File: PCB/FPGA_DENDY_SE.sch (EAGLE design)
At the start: 140 parts, among them CN1 DENDY60PINSLOT, J1 NTSC/PAL, J2 DENDY, Q1 14.318 MHz, Q2 17.734 MHz, U1 EP1C3T100C8N, U10 OPA2134U, U11 SN74LVC2G34DBVR, U12 THS7314DR, U13 74LS373WMSO20, U14 SN74LVC1G125DBVR, U15 74LVC1G04GV, U16 SN74LVC1G3157, U2 EPCS4, U3 SN74LVC8T245, U4 SN74LVC8T245, U5 SN74LVC1G240DBVR, U6 SN74LVC1G240DBVR, U7 SN74LVC1G240DBVR, U8 SN74LVC1G240DBVR, X1 057-010-1

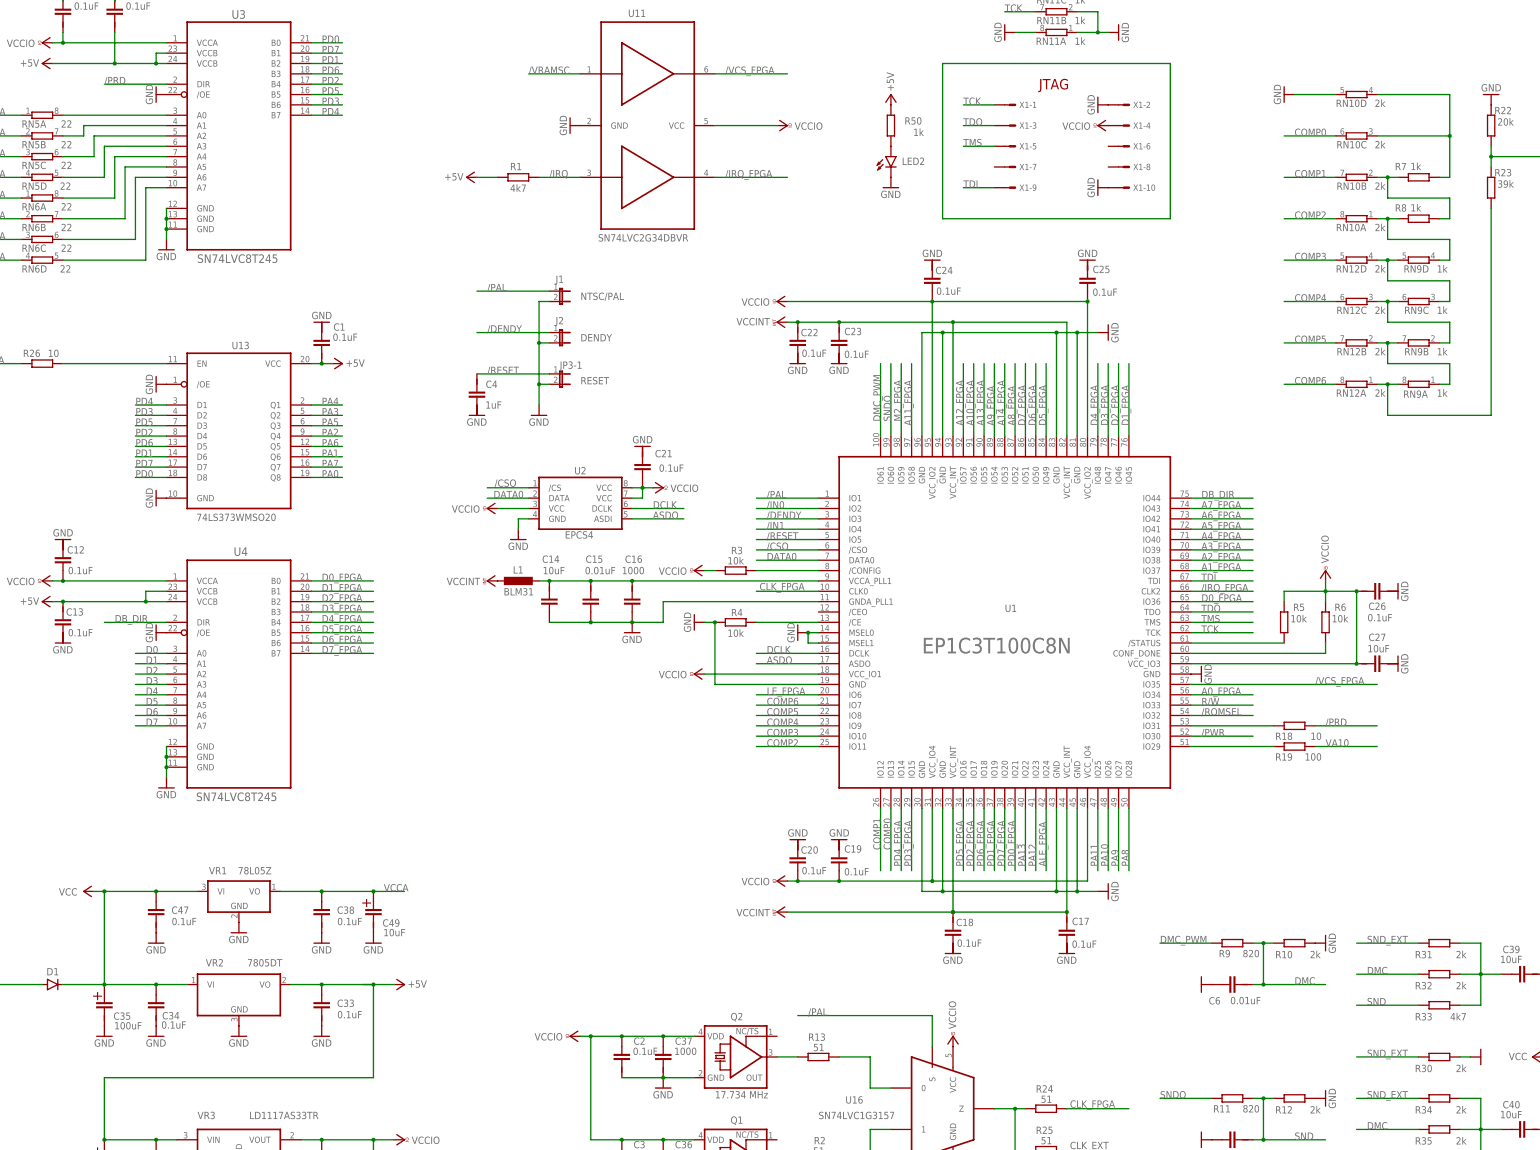
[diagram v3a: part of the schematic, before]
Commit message: Add files via upload
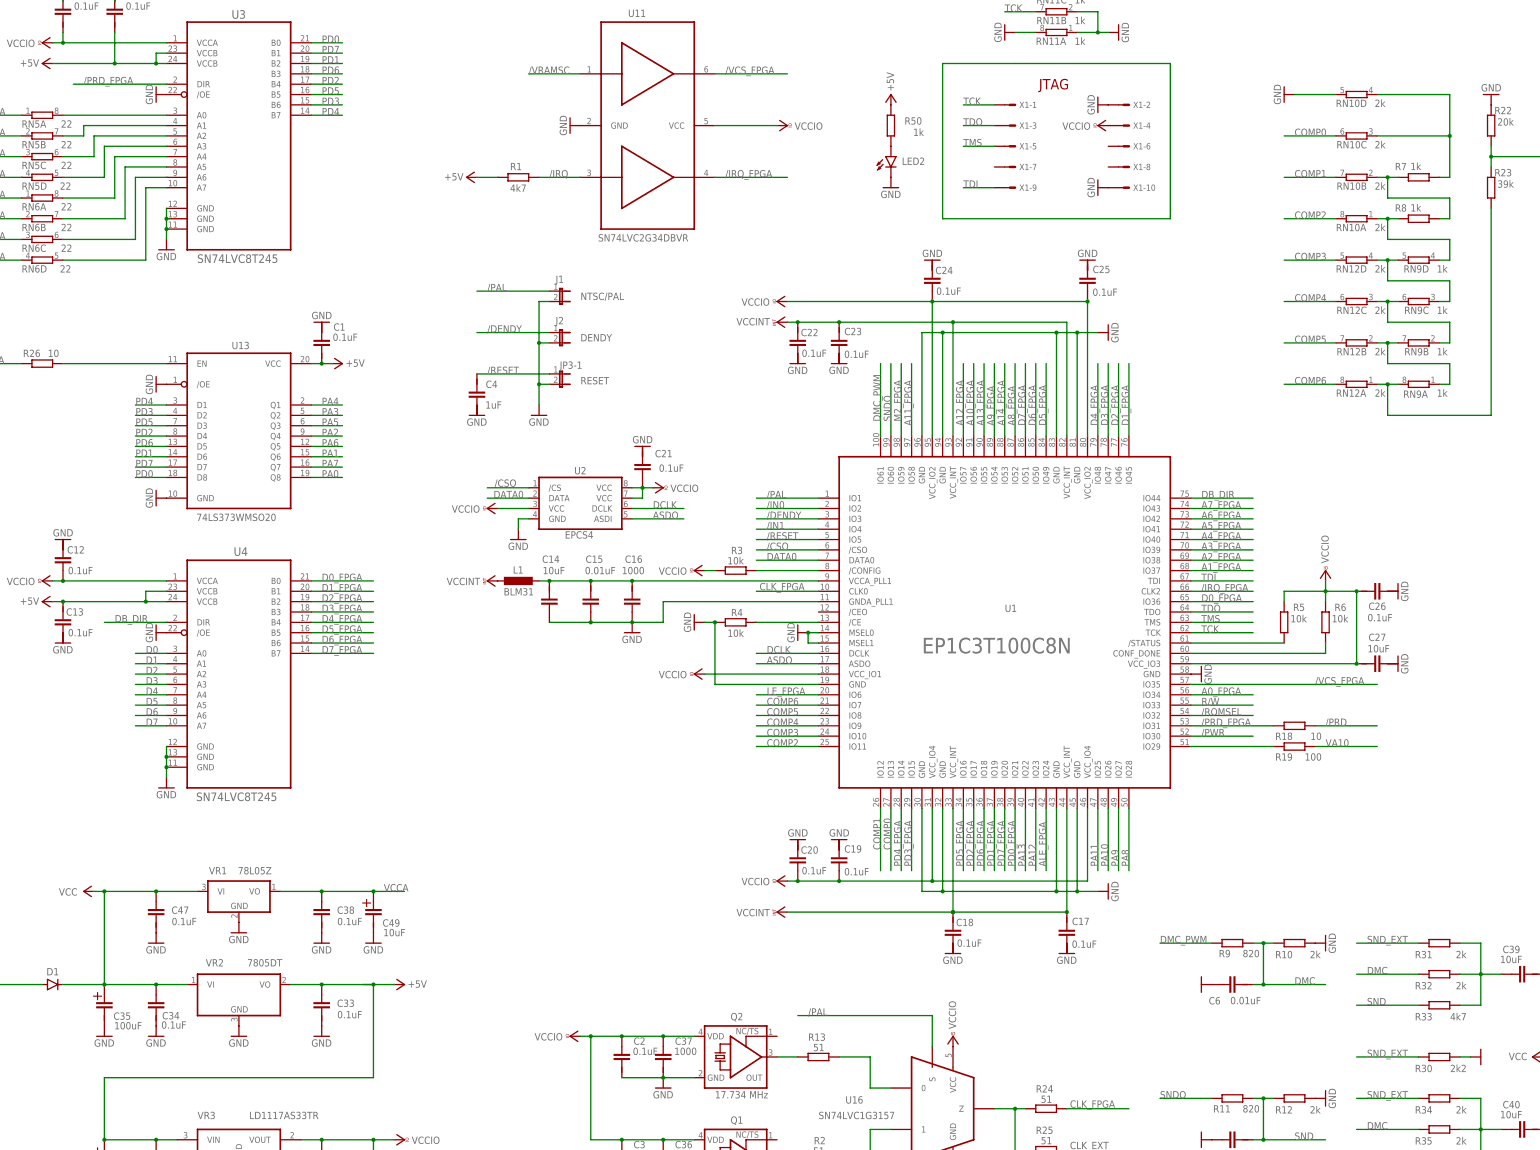
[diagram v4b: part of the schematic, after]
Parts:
- R30: value 2k -> 2k2
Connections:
- net N$14 renamed /PWR_FPGA
- removed net N$13: R18.1, U1.IO31
- new net /PRD_FPGA: R18.1, U1.IO31, U3.DIR
- net /PRD: no longer U3.DIR
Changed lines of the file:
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@@
 <part name="C5" library="rcl_my" deviceset="C-EU" device="C0805" package3d_urn="urn:adsk.eagle:package:23617/2" value="0.01uF"/>
 <part name="GND48" library="supply1" library_urn="urn:adsk.eagle:library:371" deviceset="GND" device=""/>
-<part name="R30" library="rcl" library_urn="urn:adsk.eagle:library:334" deviceset="R-EU_" device="R0805" package3d_urn="urn:adsk.eagle:package:23553/2" value="2k"/>
+<part name="R30" library="rcl" library_urn="urn:adsk.eagle:library:334" deviceset="R-EU_" device="R0805" package3d_urn="urn:adsk.eagle:package:23553/2" value="2k2"/>
 <part name="GND76" library="supply1" library_urn="urn:adsk.eagle:library:371" deviceset="GND" device=""/>
 <part name="GND49" library="supply1" library_urn="urn:adsk.eagle:library:371" deviceset="GND" device=""/>
@@
 <net name="/PRD" class="0">
 <segment>
-<pinref part="U3" gate="G$1" pin="DIR"/>
-<wire x1="-205.74" y1="129.54" x2="-220.98" y2="129.54" width="0.1524" layer="91"/>
-<label x="-220.98" y="129.54" size="1.778" layer="95"/>
-</segment>
-<segment>
 <wire x1="-350.52" y1="0" x2="-342.9" y2="0" width="0.1524" layer="91"/>
 <pinref part="CN1" gate="G$1" pin="/PRD"/>
@@
 </segment>
 </net>
-<net name="N$13" class="0">
+<net name="/PRD_FPGA" class="0">
 <segment>
 <pinref part="R18" gate="G$1" pin="1"/>
 <pinref part="U1" gate="G$1" pin="IO31"/>
 <wire x1="66.04" y1="-27.94" x2="45.72" y2="-27.94" width="0.1524" layer="91"/>
+<label x="48.26" y="-27.94" size="1.778" layer="95"/>
+</segment>
+<segment>
+<pinref part="U3" gate="G$1" pin="DIR"/>
+<wire x1="-205.74" y1="129.54" x2="-228.6" y2="129.54" width="0.1524" layer="91"/>
+<label x="-226.06" y="129.54" size="1.778" layer="95"/>
 </segment>
 </net>
-<net name="N$14" class="0">
+<net name="/PWR_FPGA" class="0">
 <segment>
 <pinref part="R19" gate="G$1" pin="1"/>

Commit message: Add files via upload
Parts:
- removed C59, C60, C61, C62: 0.1uF, rcl_my:C-EUC0805
- removed R50, R63: 1k, rcl:R-EU_R0805
- removed R67: 10, rcl:R-EU_R0805
- removed U16: SN74LVC1G3157, SN74LVC1G3157:SN74LVC1G3157
- added C51, C52, C54: 10uF, rcl_my:CPOL-EU153CLV-0505
- added C53: 0.1uF, rcl_my:C-EUC0805
- added C7: 0.1uF, rcl_my:C-EUC0603
- added R27, R28: 2k, rcl:R-EU_R0805
- added R29: 4k7, rcl:R-EU_R0805
- added U9: THS7314DR, THS7314DR:THS7314
- C10: value 0.1uF -> 10uF; device rcl_my:C-EUC0805 -> rcl_my:CPOL-EU153CLV-0505
- C11: value 220uF -> 100uF
- C12, C13, C17, C18, C50, C8: device rcl_my:C-EUC0603 -> rcl_my:C-EUC0805
- C14: value 10uF -> 100uF; device rcl_my:C-EUC0603 -> rcl_my:CPOL-EU153CLV-0505
- C15: value 0.01uF -> 0.1uF; device rcl_my:C-EUC0603 -> rcl_my:C-EUC0805
- C16: value 1000 -> 0.1uF; device rcl_my:C-EUC0603 -> rcl_my:C-EUC0805
- C19: value 0.1uF -> 22uF; device rcl_my:C-EUC0603 -> rcl_my:CPOL-EU153CLV-0505
- C26: value 0.1uF -> 10uF
- C27: value 10uF -> 0.01uF
- C28: value 0.1uF -> 1000; device rcl_my:C-EUC0805 -> rcl_my:C-EUC0603
- C29: value 0.1uF -> 1uF; device rcl_my:C-EUC0805 -> rcl_my:C-EUC0603
- C30, C31, C33, C38, C40, C45: device rcl_my:C-EUC0805 -> rcl_my:C-EUC0603
- C32: value 22uF -> 0.1uF; device rcl_my:CPOL-EU153CLV-0505 -> rcl_my:C-EUC0603
- C35: value 100uF -> 1000; device rcl_my:CPOL-EU153CLV-0505 -> rcl_my:C-EUC0805
- C36: value 1000 -> 0.1uF
- C39: value 10uF -> 0.1uF; device rcl_my:C-EUC0805 -> rcl_my:C-EUC0603
- C4: value 1uF -> 0.1uF; device rcl_my:C-EUC0603 -> rcl_my:C-EUC0805
- C41, C42: value 0.1uF -> 0.01uF
- C43: value 10uF -> 0.1uF; device rcl_my:CPOL-EU153CLV-0505 -> rcl_my:C-EUC0603
- C44: value 10uF -> 220uF
- C46: value 10uF -> 0.1uF
- C48: value 0.1uF -> 10uF; device rcl_my:C-EUC0603 -> rcl_my:C-EUC0805
- C49: device rcl_my:CPOL-EU153CLV-0505 -> rcl_my:C-EUC0805
- C5: value 0.01uF -> 0.1uF
- C6: value 0.01uF -> 0.1uF; device rcl_my:C-EUC0805 -> rcl_my:C-EUC0603
- C9: value 100uF -> 0.1uF; device rcl_my:CPOL-EU153CLV-0505 -> rcl_my:C-EUC0805
- R1: value 4k7 -> 10
- R10: value 2k -> 51
- R11: value 820 -> 1k
- R12: value 2k -> 1k
- R13: value 51 -> 20k
- R14: value 10k -> 39k
- R17: value 10k -> 10
- R18: value 10 -> 100
- R19: value 100 -> 820
- R2: value 51 -> 10
- R20: value 10 -> 2k
- R21: value 75 -> 820
- R22: value 20k -> 2k
- R23: value 39k -> 2k
- R24: value 51 -> 2k
- R25: value 51 -> 4k7
- R26: value 10 -> 2k2
- R3: value 10k -> 4k7
- R30: value 2k2 -> 75
- R31, R32, R34: value 2k -> 10k
- R33: value 4k7 -> 10k
- R35: value 2k -> 10
- R36, RN8: value 4k7 -> 1k
- R4: value 10k -> 1k
- R7, R8: value 1k -> 51
- R9: value 820 -> 51
- RN12: value 2k -> 4k7
- RN9: value 1k -> 2k
- U10: value OPA2134U -> SN74LVC1G125DBVR; device burr-brown:OPA2134U -> SN74LVC1G125DBVR:SN74LVC1G125DBVR
- U11: value SN74LVC2G34DBVR -> SN74LVC1G240DBVR; device SN74LVC2G34DBVR:SN74LVC2G34DBVR -> SN74LVC1G240DBVR:SN74LVC1G240DBVR
- U12: value THS7314DR -> SN74LVC1G240DBVR; device THS7314DR:THS7314 -> SN74LVC1G240DBVR:SN74LVC1G240DBVR
- U13: value 74LS373WMSO20 -> SN74LVC1G240DBVR; device 74LS373WM:74LS373WMSO20 -> SN74LVC1G240DBVR:SN74LVC1G240DBVR
- U14: value SN74LVC1G125DBVR -> SN74LVC1G240DBVR; device SN74LVC1G125DBVR:SN74LVC1G125DBVR -> SN74LVC1G240DBVR:SN74LVC1G240DBVR
- U15: value 74LVC1G04GV -> OPA2134U; device 74LVC1G04GV:74LVC1G04GV -> burr-brown:OPA2134U
- U2: value EPCS4 -> SN74LVC8T245; device EPCS4:EPCS4 -> SnapEDA-Library:SN74LVC8T245
- U3: value SN74LVC8T245 -> 74LS373WMSO20; device SnapEDA-Library:SN74LVC8T245 -> 74LS373WM:74LS373WMSO20
- U5: value SN74LVC1G240DBVR -> SN74LVC2G34DBVR; device SN74LVC1G240DBVR:SN74LVC1G240DBVR -> SN74LVC2G34DBVR:SN74LVC2G34DBVR
- U6: value SN74LVC1G240DBVR -> 74LVC1G04GV; device SN74LVC1G240DBVR:SN74LVC1G240DBVR -> 74LVC1G04GV:74LVC1G04GV
- U7: value SN74LVC1G240DBVR -> EPCS4; device SN74LVC1G240DBVR:SN74LVC1G240DBVR -> EPCS4:EPCS4
- U8: value SN74LVC1G240DBVR -> SN74LVC1G3157; device SN74LVC1G240DBVR:SN74LVC1G240DBVR -> SN74LVC1G3157:SN74LVC1G3157
- renumbered R61 to R39, R62 to R40, R64 to R41, R65 to R37, R66 to R42, R68 to R38
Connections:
- net +5V: now also C13.1, C14.+, C15.1, C2.1, C20.2, C4.2, C45.2, C46.1, C47.1, C5.2, C7.2, R3.1, R31.1, R32.1, R33.1, R34.1, R4.2, U10.VCC, U11.VCC, U12.VCC, U2.VCCB@1, U2.VCCB@2, U3.VCC; no longer C10.2, C13.2, C28.1, C33.1, C50.2, C59.2, C60.1, C61.1, C62.1, C8.2, C9.+, R1.1, R14.1, R15.1, R16.1, R17.1, R50.2, U15.VCC, U3.VCCB@1, U3.VCCB@2, U5.VCC, U7.VCC, U8.VCC
- net /CSO: now also U7./CS; no longer U2./CS
- net /IN0: now also U11./OE, U13./OE; no longer U6./OE, U8./OE
- net /IN1: now also U12./OE, U14./OE; no longer U5./OE, U7./OE
- net /IRQ: now also R3.2, U5.IN2; no longer R1.2, U11.IN2
- net /IRQ_FPGA: now also U5.OUT2; no longer U11.OUT2
- net /PA13: now also U6.OUT; no longer U15.OUT
- net /PAL: now also U8.S; no longer U16.S
- net /PRD: now also R17.2; no longer R18.2
- net /PRD_FPGA: now also R17.1, U2.DIR; no longer R18.1, U3.DIR
- net /PWR_FPGA: now also R18.1; no longer R19.1
- net /RESET: now also C29.2; no longer C4.2
- net /VCS_FPGA: now also U5.OUT1; no longer U11.OUT1
- net /VRAMSC: now also U5.IN1; no longer U11.IN1
- net ALE_FPGA: now also R2.1; no longer R26.1
- net ASDO: now also U7.ASDI; no longer U2.ASDI
- net CLK_EXT: now also R10.2; no longer R25.2
- net CLK_FPGA: now also R9.2; no longer R24.2
- net COMP0: now also RN9C.2; no longer RN10C.2
- net COMP1: now also RN9B.2; no longer RN10B.2
- net COMP2: now also RN9A.2; no longer RN10A.2
- net COMP3: now also RN10D.2; no longer RN12D.2
- net COMP4: now also RN10C.2; no longer RN12C.2
- net COMP5: now also RN10B.2; no longer RN12B.2
- net COMP6: now also RN10A.2; no longer RN12A.2
- net D0: now also U13.Y, U14.Y; no longer U5.Y, U6.Y
- net DATA0: now also U7.DATA; no longer U2.DATA
- net DCLK: now also U7.DCLK; no longer U2.DCLK
- net DMC: now also C41.2, R19.2, R20.1, R24.1, R28.1; no longer C6.2, R10.1, R32.1, R35.1, R9.2
- net DMC_PWM: now also R19.1; no longer R9.1
- net GND: now also C10.-, C11.-, C12.2, C13.2, C14.-, C15.2, C16.2, C17.2, C18.2, C26.1, C27.1, C28.1, C35.2, C42.1, C53.2, C54.-, C8.2, C9.2, R13.2, R20.2, R26.2, R6.1, RN12A.1, RN12D.1, RN8A.2, RN8B.1, RN9D.2, U10./OE, U15A.V-, U2./OE, U2.GND@1, U2.GND@2, U2.GND@3, U3.GND, U5.GND, U6.GND, U7.GND, U8.GND, U9.GND; no longer C10.1, C14.1, C15.1, C16.1, C2.2, C28.2, C29.2, C3.2, C30.2, C31.2, C33.2, C35.-, C38.2, C45.2, C49.-, C5.1, C6.1, C60.2, C61.2, C62.2, C9.-, R10.2, R12.2, R30.2, R4.1, RN10D.2, RN11A.1, RN11A.2, RN11B.1, RN8D.1, U10A.V-, U11.GND, U12.GND, U13./OE, U13.GND, U14./OE, U15.GND, U16.GND, U2.GND, U3.GND@1, U3.GND@2, U3.GND@3
- net JOYDATA1: now also R31.2, U13.A; no longer R14.2, U6.A
- net JOYDATA2: now also R33.2, U14.A; no longer R15.2, U5.A
- net LCH: now also C52.-; no longer C44.-
- net LE: now also U10.Y; no longer U14.Y
- net LE_FPGA: now also U10.A; no longer U14.A
- net M2_FPGA: now also U11.A, U12.A; no longer U7.A, U8.A
- net N$1: now also R15.1; no longer R5.1
- net N$10: now also R6.2; no longer R4.2
- net N$11: now also R5.2; no longer R3.2
- net N$12: now also C26.2, C27.2, C28.2; no longer C14.2, C15.2, C16.2
- net N$16: now also C48.1, R23.2, R24.2, R25.2; no longer C39.1, R31.2, R32.2, R33.2
- net N$17: now also R8.1; no longer R2.1
- net N$18: now also R7.1; no longer R13.1
- net N$19: now also U2.A1; no longer U3.A1
- net N$2: now also R16.1; no longer R6.1
- net N$20: now also U2.A2; no longer U3.A2
- net N$21: now also U2.A3; no longer U3.A3
- net N$22: now also U2.A4; no longer U3.A4
- net N$23: now also U2.A5; no longer U3.A5
- net N$24: now also U2.A6; no longer U3.A6
- net N$25: now also U2.A7; no longer U3.A7
- net N$26: now also R11.1, R12.2, RN9B.1; no longer R7.1, R8.2, RN10B.1
- net N$28: now also R14.1, RN10A.1, RN11A.2; no longer R23.1, RN12A.1, RN9A.2
- net N$30: now also C49.1, R27.2, R28.2, R29.2; no longer C40.1, R34.2, R35.2, R36.2
- net N$33: now also R1.1; no longer R20.1
- net N$34: now also R30.1, U9.CH3_OUT; no longer R21.1, U12.CH3_OUT
- net N$35: now also R7.2, U8.0; no longer R13.2, U16.0
- net N$36: now also C44.+, R30.2; no longer C11.+, R21.2
- net N$37: now also C51.+, R35.2; no longer C43.+, R67.2
- net N$38: now also C48.2, RN12C.1, RN12D.2, U15A.+IN; no longer C39.2, RN8C.1, RN8D.2, U10A.+IN
- net N$39: now also C49.2, RN12A.2, RN12B.1, U15B.+IN; no longer C40.2, RN8A.2, RN8B.1, U10B.+IN
- net N$4: now also RN10B.1, RN11A.1, RN11B.2; no longer RN12B.1, RN9A.1, RN9B.2
- net N$40: now also RN10D.1, RN11C.1, RN11D.2; no longer RN12D.1, RN9C.1, RN9D.2
- net N$41: now also R13.1, R14.2, U9.CH1_IN, U9.CH2_IN, U9.CH3_IN; no longer R22.1, R23.2, U12.CH1_IN, U12.CH2_IN, U12.CH3_IN
- net N$42: now also R36.2, U15A.-IN; no longer R63.2, U10A.-IN
- net N$43: now also R35.1, U15A.OUT; no longer R67.1, U10A.OUT
- net N$44: now also U15B.OUT; no longer U10B.OUT
- net N$45: now also U15B.-IN; no longer U10B.-IN
- net N$46: now also R8.2, U8.1; no longer R2.2, U16.1
- net N$47: now also R10.1, R9.1, U8.Z; no longer R24.1, R25.1, U16.Z
- net N$48: now also C52.+; no longer C44.+
- net N$5: now also R11.2, RN9C.1, RN9D.1; no longer R7.2, RN10C.1, RN10D.1
- net N$6: now also R2.2, U3.EN; no longer R26.2, U13.EN
- net N$63: now also R4.1; no longer R50.1
- net N$7: now also U2.A0; no longer U3.A0
- net N$8: now also R12.1, RN11D.1, RN9A.1; no longer R8.1, RN10A.1, RN9D.1
- net N$9: now also RN10C.1, RN11B.1, RN11C.2; no longer RN12C.1, RN9B.1, RN9C.2
- net PA0: now also U3.Q8; no longer U13.Q8
- net PA1: now also U3.Q6; no longer U13.Q6
- net PA12: now also R1.2; no longer R20.2
- net PA13: now also U6.IN; no longer U15.IN
- net PA2: now also U3.Q4; no longer U13.Q4
- net PA3: now also U3.Q2; no longer U13.Q2
- net PA4: now also U3.Q1; no longer U13.Q1
- net PA5: now also U3.Q3; no longer U13.Q3
- net PA6: now also U3.Q5; no longer U13.Q5
- net PA7: now also U3.Q7; no longer U13.Q7
- net PD0: now also U2.B0, U3.D8; no longer U13.D8, U3.B0
- net PD1: now also U2.B2, U3.D6; no longer U13.D6, U3.B2
- net PD2: now also U2.B4, U3.D4; no longer U13.D4, U3.B4
- net PD3: now also U2.B6, U3.D2; no longer U13.D2, U3.B6
- net PD4: now also U2.B7, U3.D1; no longer U13.D1, U3.B7
- net PD5: now also U2.B5, U3.D3; no longer U13.D3, U3.B5
- net PD6: now also U2.B3, U3.D5; no longer U13.D5, U3.B3
- net PD7: now also U2.B1, U3.D7; no longer U13.D7, U3.B1
- net RCH: now also C51.-; no longer C43.-
- net SCK1: now also R32.2, U11.Y; no longer R16.2, U8.Y
- net SCK2: now also R34.2, U12.Y; no longer R17.2, U7.Y
- net SND: now also C42.2, R21.2, R22.1, R25.1, R29.1; no longer C5.2, R11.2, R12.1, R33.1, R36.1
- net SNDO: now also R21.1; no longer R11.1
- net SND_EXT: now also R23.1, R26.1, R27.1; no longer R30.1, R31.1, R34.1
- net TCK: now also RN8B.2; no longer RN11B.2
- net TDI: now also RN8D.2; no longer RN11D.2
- net TMS: now also RN8C.2; no longer RN11C.2
- net VA10: now also R18.2; no longer R19.2
- net VCC: now also C11.+, C12.1, C50.2, C8.1, RN12B.2, RN12C.2, U15A.V+; no longer C34.1, C35.+, C42.2, C47.1, RN8B.2, RN8C.2, U10A.V+
- net VCCA: now also C10.+, C43.2, C9.1, U9.VS+; no longer C38.1, C48.2, C49.+, U12.VS+
- net VCCINT: now also C18.1, C19.+, C32.2, C33.2; no longer C17.2, C18.2, C31.1, C32.+
- net VCCIO: now also C16.1, C17.1, C3.2, C31.1, C34.1, C35.1, C38.2, C39.2, C40.2, C6.1, R15.2, R16.2, R5.1, RN8C.1, RN8D.1, U2.VCCA, U5.VCC, U7.VCC@1, U7.VCC@2, U7.VCC@3, U8.VCC; no longer C12.1, C19.1, C2.1, C20.1, C26.2, C27.2, C29.1, C3.1, C41.2, R3.1, R5.2, R6.2, RN11C.1, RN11D.1, U11.VCC, U16.VCC, U2.VCC@1, U2.VCC@2, U2.VCC@3, U3.VCCA
- net VIDEO: now also C44.-; no longer C11.-
- net VPPL3: now also C53.1, C54.+, R36.1; no longer C45.1, C46.1, R63.1
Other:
- moved on the sheet: C1, C11, C12, C13, C15, C16, C17, C18, C2, C20, C26, C27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

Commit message: Add files via upload
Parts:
- D1: value (none) -> 1N4007(M7)
- J1: value NTSC/PAL -> /PAL
- J2: value DENDY -> /DENDY
- JP1: value (none) -> PWR_ON
- JP3: value (none) -> #RESET
- LED2: value (none) -> GNL-1206YC
- R4: value 1k -> 1k2
- X2: value (none) -> JOYPAD1
- X3: value (none) -> 9V
- X4: value (none) -> JOYPAD2
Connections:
- net GND: now also C1.1, C19.-, C2.2, C20.1, C21.2, C22.1, C23.1, C24.2, C25.2, C29.1, C3.1, C30.2, C31.2, C32.1, C33.1, C38.1, C39.1, C4.1, C40.1, C43.1, C45.1, C5.1, C50.1, C6.2, C7.1, U10.GND, U11.GND, U12.GND, U13.GND, U14.GND, VR3.GND, VR4.GND
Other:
- note removed: "JOYPAD 1"
- note removed: "JOYPAD 2"
- note removed: "PWR ON"
- note removed: "RESET"
- moved on the sheet: JP1-1, X3

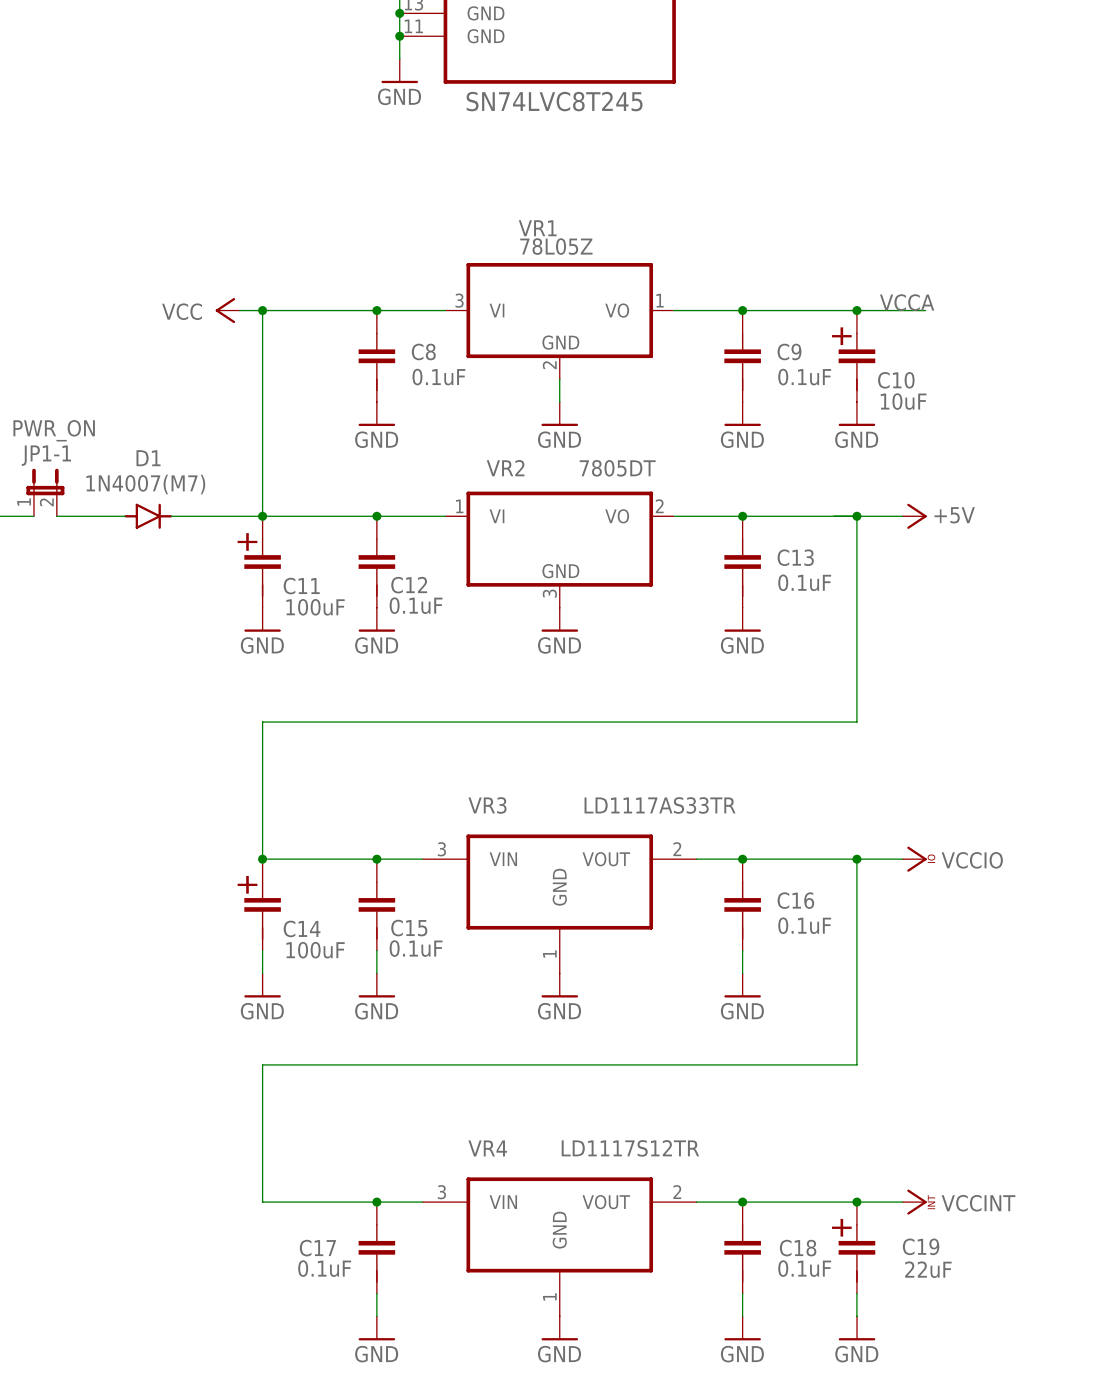
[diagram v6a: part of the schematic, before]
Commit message: Add files via upload
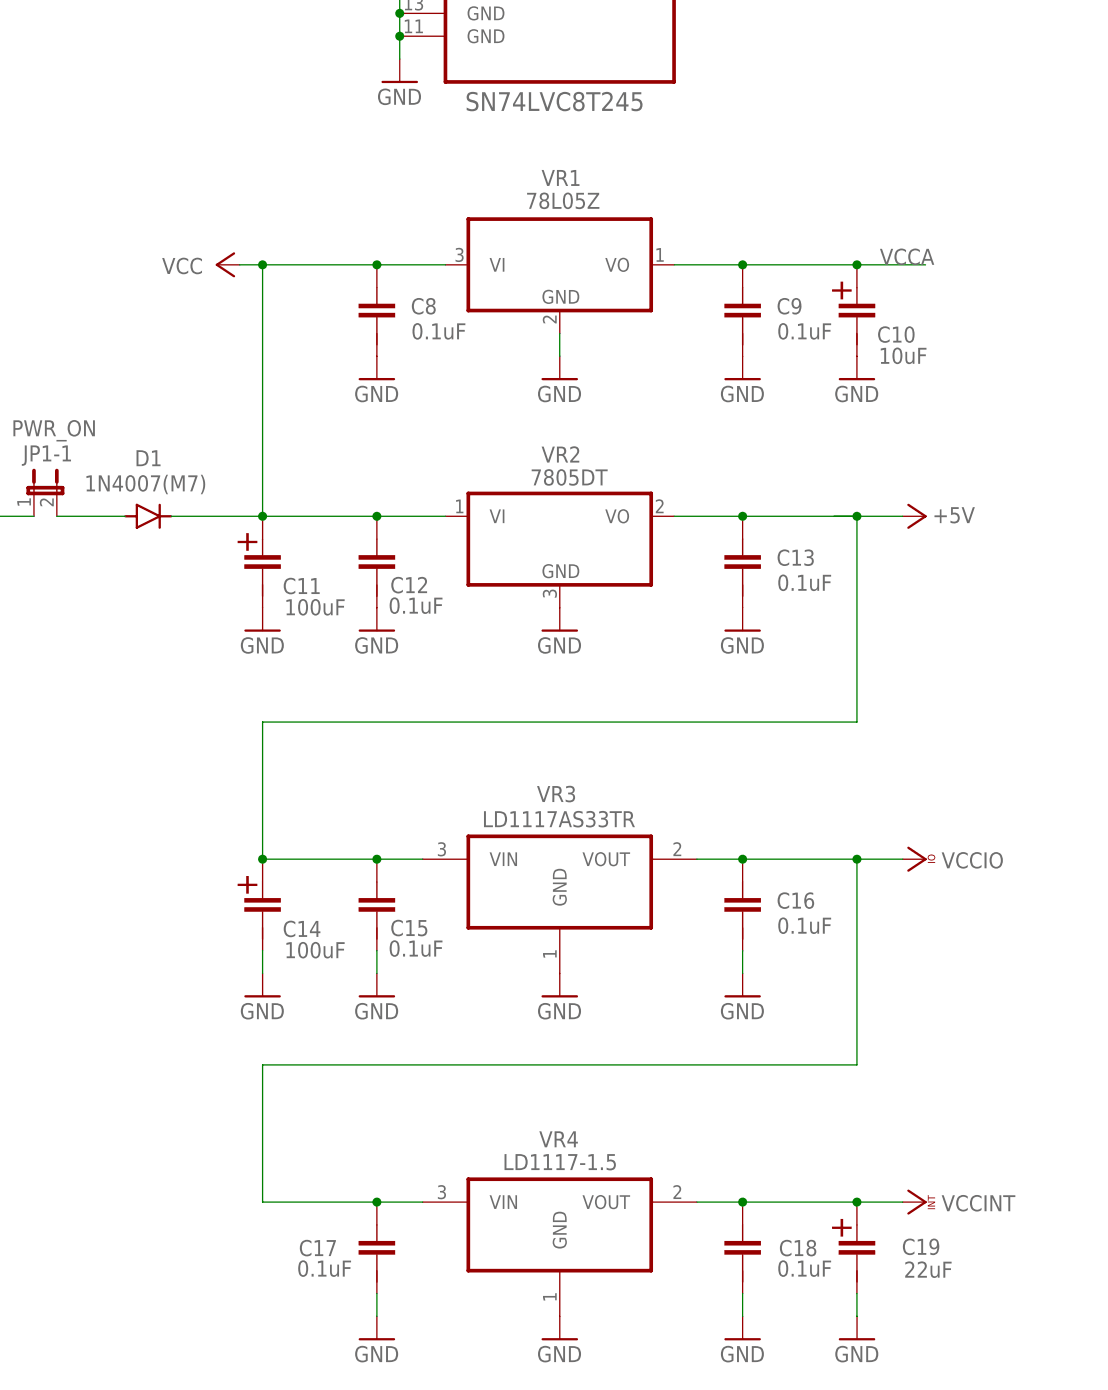
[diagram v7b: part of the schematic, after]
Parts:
- VR4: value LD1117S12TR -> LD1117-1.5; device LD1117S12TR:LD1117S12TR -> LD1117-1.5:LD1117-1.5
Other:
- moved on the sheet: C10, C8, C9, VR1
